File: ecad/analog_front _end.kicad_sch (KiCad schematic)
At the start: 26 parts, among them J3 Red Banana Plug, J4 Black Banana Plug, SW3 GF-126-0159, SW4 GF-123-0054, U10 MCP3561, U3 OPA4388IDR, U7 LM4030-2.5

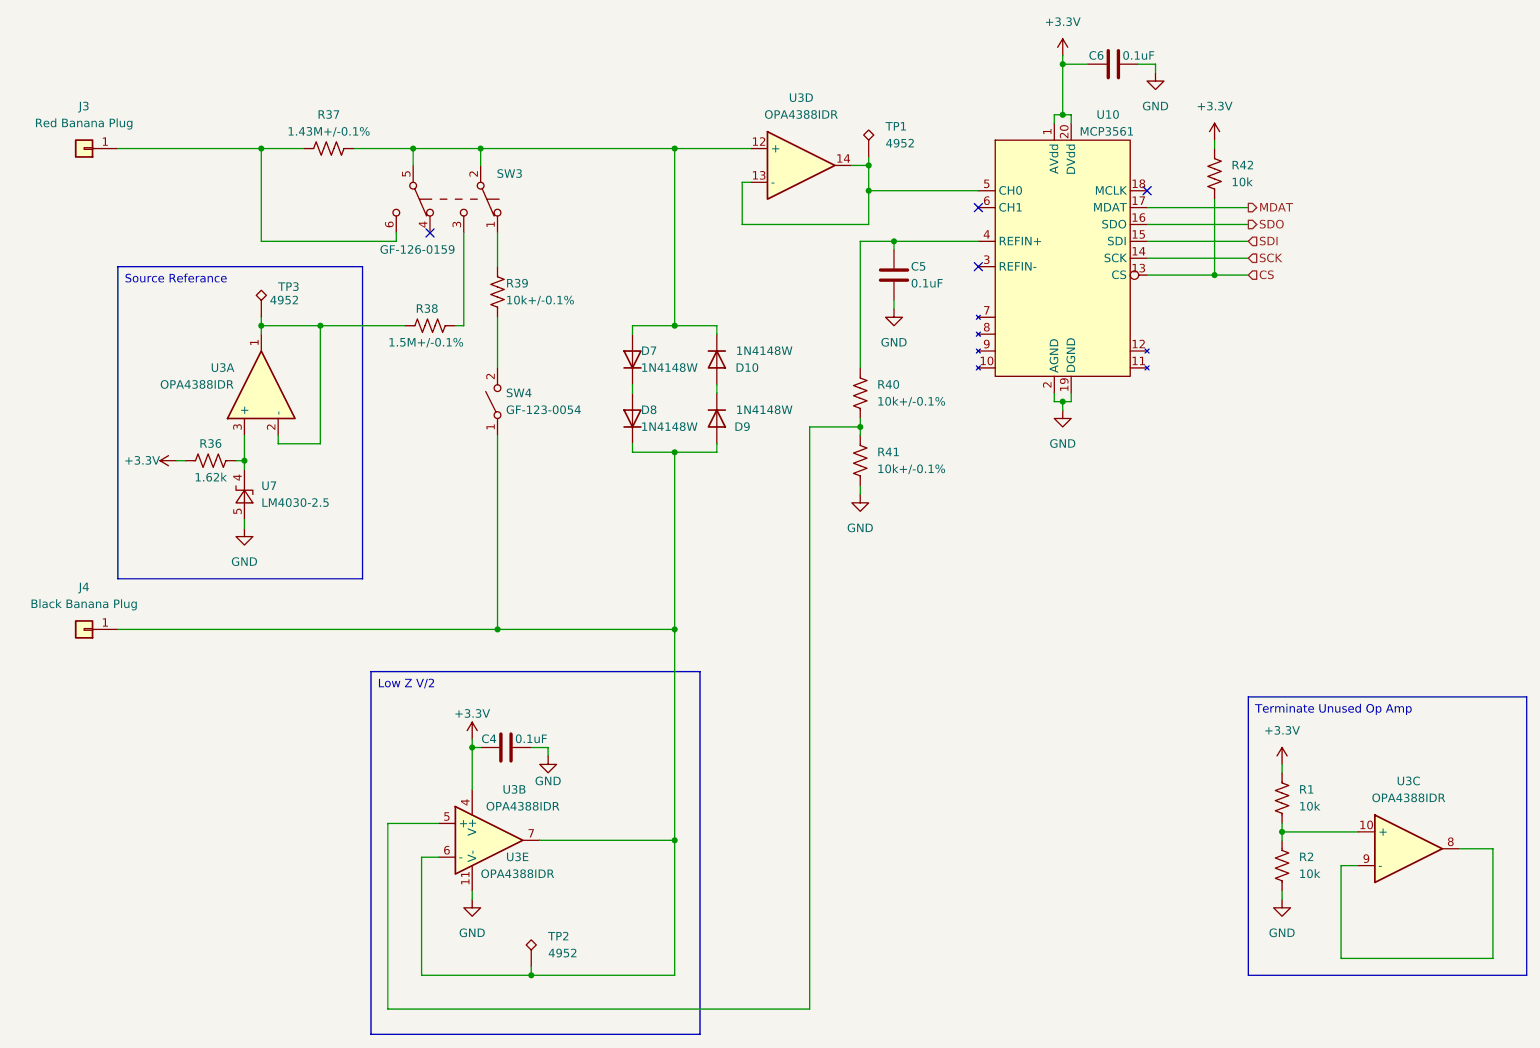
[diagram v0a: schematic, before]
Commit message: layout finished
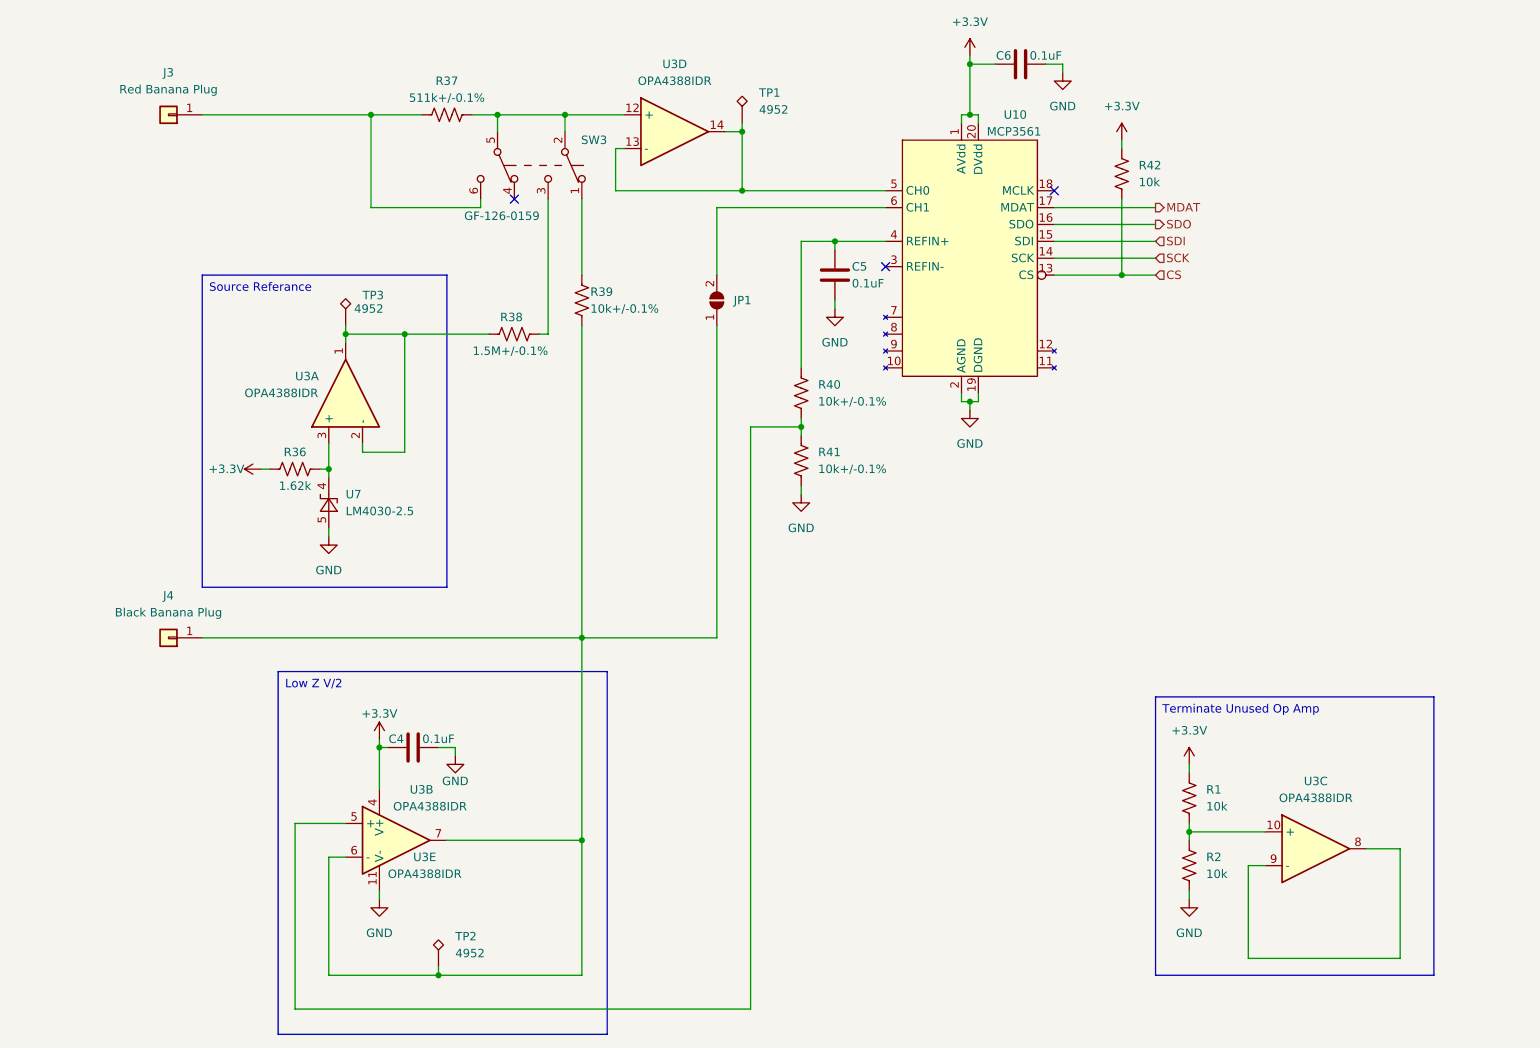
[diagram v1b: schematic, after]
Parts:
- removed D10, D7, D8, D9: 1N4148W, Diode_SMD:D_SOD-123, symbol Diode:1N4148W
- removed SW4: GF-123-0054, Multimeter:SW_GF-123-0054, symbol Switch:SW_SPST
- added JP1: ~, Jumper:SolderJumper-2_P1.3mm_Open_Pad1.0x1.5mm, symbol Jumper:SolderJumper_2_Open
- C4, C5, C6: Digikey Part # (none) -> 1276-1003-1-ND; Part # (none) -> CL21B104KBCNNNC; Unit Price (none) -> 0.1
- J3, J4: Digikey Part # (none) -> 36-575-8-ND; Part # (none) -> 575-8; Unit Price (none) -> 0.88
- R1, R2, R42: Digikey Part # (none) -> RMCF0805FT10K0CT-ND; Part # (none) -> RMCF0805FT10K0; Unit Price (none) -> 0.1
- R36: Digikey Part # (none) -> RMCF0805FT1K62CT-ND; Part # (none) -> RMCF0805FT1K62; Unit Price (none) -> 0.1
- R37: value 1.43M+/-0.1% -> 511k+/-0.1%; Digikey Part # (none) -> P511KDACT-ND; Part # (none) -> ERA-6AEB5113V
- R38: Digikey Part # (none) -> 408-2025-1-ND; Part # (none) -> RG2012P-155-B-T5; Unit Price (none) -> 0.1
- R39, R40, R41: Digikey Part # (none) -> P10KDACT-ND; Part # (none) -> ERA-6AEB103V; Unit Price (none) -> 0.32
- SW3: Digikey Part # (none) -> SW342-ND; Part # (none) -> GF-126-0159; Unit Price (none) -> 1.58
- TP1, TP2, TP3: Digikey Part # (none) -> 36-4952-ND; Part # (none) -> 4952; Unit Price (none) -> 0.26
- U10: Digikey Part # (none) -> 150-MCP3561RT-E/STCT-ND; Part # (none) -> MCP3561RT-E/ST; Unit Price (none) -> 3.00
- U3: Digikey Part # (none) -> 296-53511-1-ND; Part # (none) -> OPA4388IDR; Unit Price (none) -> 4.92
- U7: Digikey Part # (none) -> LM4030CMF-2.5/NOPBCT-ND; Part # (none) -> LM4030CMF-2.5/NOPB; Unit Price (none) -> 1.61
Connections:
- net at J4.1 (Pin_1), TP2.1, U3.6 (-)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: now also R39.2, JP1.1 (A)
- net at U10.6 (CH1): now also JP1.2 (B)
- no-connect marks 4 -> 3
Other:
- moved on the sheet: C4, C5, C6, J3, J4, R1, R2, R36, R37, R38, R39, R40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
